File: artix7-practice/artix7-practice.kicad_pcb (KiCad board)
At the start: 2 copper layers, 20.3 x 8.4 mm, 73 parts, among them J101 USB_B_Micro, J102 Conn_02x06_Odd_Even, J103 Bus_PCI_Express_x1, Q101 Q_NMOS_GSD, U101 XC7A35T-FTG256, U104 FT2232HL, U105 93CxxC, U106 W25Q128JVS, U108 LMR33630ADDA, U109 LMR33630ADDA, U110 LMR33630ADDA, X101 125MHz, Y101 ABM8-272-T3

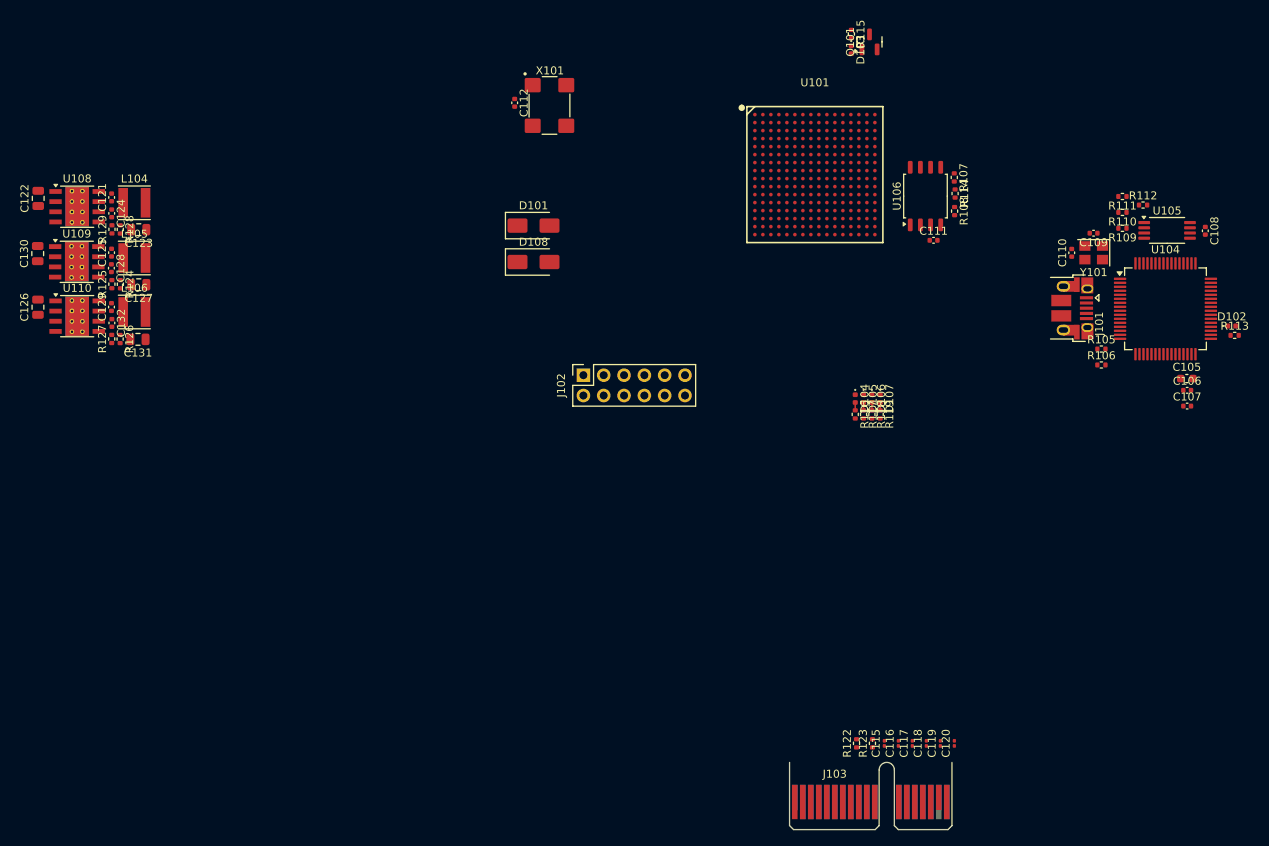
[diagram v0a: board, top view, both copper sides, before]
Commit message: JLCPCB uploads
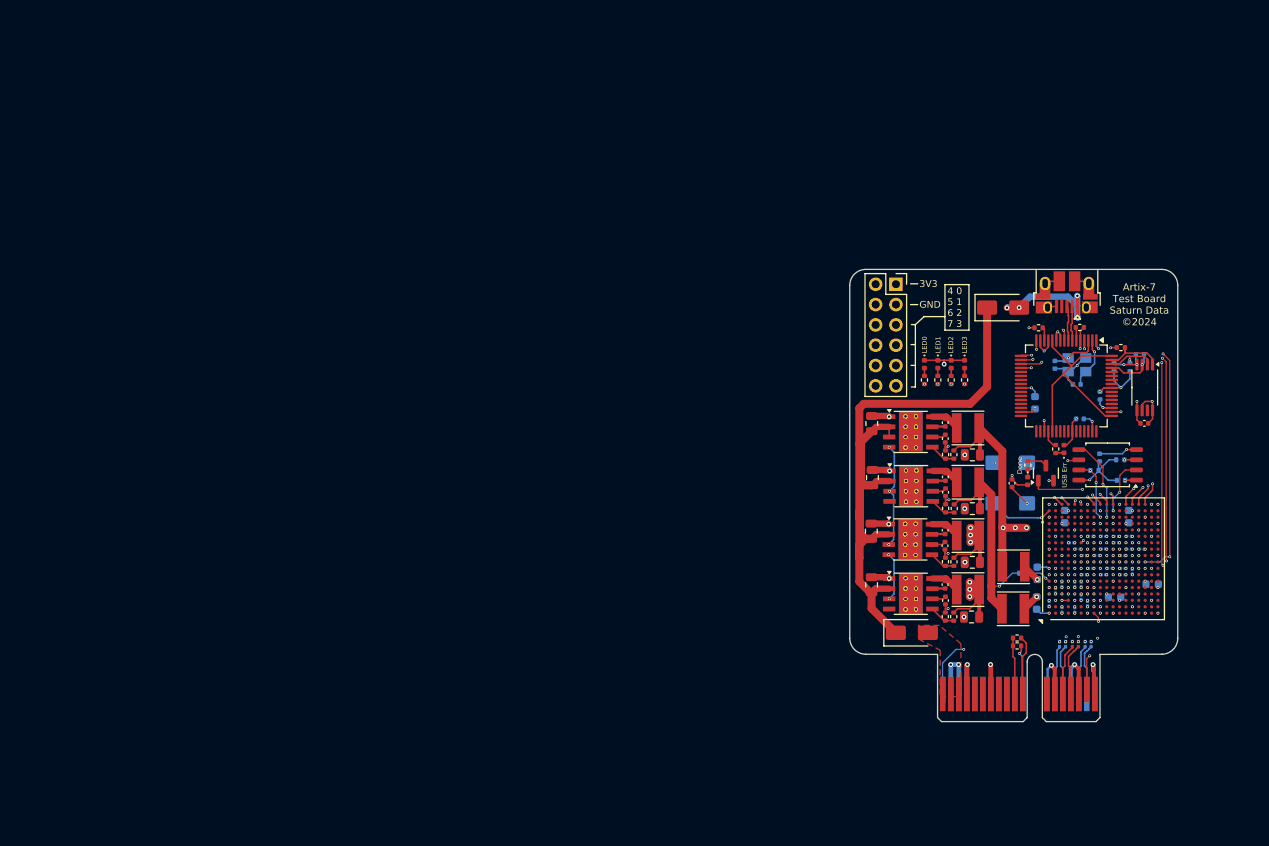
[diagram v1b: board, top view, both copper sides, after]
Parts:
- added C101: 100n, Capacitor_SMD:C_0402_1005Metric, F.Cu at (71.0, 77.8)
- added C102: 22u, Capacitor_SMD:C_0805_2012Metric, F.Cu at (61.8, 77.9)
- added C103: 22u, Capacitor_SMD:C_0805_2012Metric, F.Cu at (74.3, 81.8)
- added C104: 1u, Capacitor_SMD:C_0402_1005Metric, F.Cu at (71.0, 79.8)
- added C113: 22u, Capacitor_SMD:C_0603_1608Metric, B.Cu at (82.4, 89.9)
- added C114: 22u, Capacitor_SMD:C_0603_1608Metric, B.Cu at (82.4, 93.6)
- added C133: 1u, Capacitor_SMD:C_0201_0603Metric, B.Cu at (87.9, 91.3)
- added C134: 1u, Capacitor_SMD:C_0201_0603Metric, B.Cu at (88.7, 93.7)
- added C135: 1u, Capacitor_SMD:C_0201_0603Metric, B.Cu at (85.5, 94.5)
- added C136: 1u, Capacitor_SMD:C_0201_0603Metric, B.Cu at (84.7, 92.1)
- added C137: 1u, Capacitor_SMD:C_0201_0603Metric, B.Cu at (85.5, 91.3)
- added C138: 100n, Capacitor_SMD:C_0201_0603Metric, B.Cu at (87.1, 91.3)
- added C139: 1u, Capacitor_SMD:C_0201_0603Metric, B.Cu at (93.9, 86.9)
- added C140: 100n, Capacitor_SMD:C_0201_0603Metric, B.Cu at (87.1, 94.5)
- added C141: 100n, Capacitor_SMD:C_0201_0603Metric, B.Cu at (83.9, 93.7)
- added C142: 1u, Capacitor_SMD:C_0201_0603Metric, B.Cu at (87.9, 92.9)
- added C143: 1u, Capacitor_SMD:C_0201_0603Metric, B.Cu at (90.7, 86.9)
- added C144: 100n, Capacitor_SMD:C_0201_0603Metric, B.Cu at (93.1, 87.7)
- added C145: 100n, Capacitor_SMD:C_0201_0603Metric, B.Cu at (88.3, 87.7)
- added C146: 1u, Capacitor_SMD:C_0201_0603Metric, B.Cu at (87.5, 86.9)
- added C147: 1u, Capacitor_SMD:C_0201_0603Metric, B.Cu at (89.1, 89.3)
- added C148: 100n, Capacitor_SMD:C_0201_0603Metric, B.Cu at (93.1, 90.1)
- added C149: 100n, Capacitor_SMD:C_0201_0603Metric, B.Cu at (88.3, 90.1)
- added C150: 1u, Capacitor_SMD:C_0201_0603Metric, B.Cu at (93.1, 89.3)
- added C151: 1u, Capacitor_SMD:C_0201_0603Metric, B.Cu at (91.5, 89.3)
- added C152: 100n, Capacitor_SMD:C_0201_0603Metric, B.Cu at (90.7, 90.1)
- added C153: 100n, Capacitor_SMD:C_0201_0603Metric, B.Cu at (92.3, 86.1)
- added C154: 1u, Capacitor_SMD:C_0201_0603Metric, B.Cu at (89.1, 85.3)
- added C155: 1u, Capacitor_SMD:C_0201_0603Metric, B.Cu at (90.7, 85.3)
- added C156: 1u, Capacitor_SMD:C_0201_0603Metric, B.Cu at (93.9, 85.3)
- added C157: 100n, Capacitor_SMD:C_0201_0603Metric, B.Cu at (92.3, 85.3)
- added C158: 1u, Capacitor_SMD:C_0201_0603Metric, B.Cu at (89.9, 87.7)
- added C159: 1u, Capacitor_SMD:C_0201_0603Metric, B.Cu at (95.5, 86.9)
- added C160: 1u, Capacitor_SMD:C_0201_0603Metric, B.Cu at (86.7, 86.1)
- added C161: 1u, Capacitor_SMD:C_0201_0603Metric, B.Cu at (94.3, 89.7)
- added C162: 22u, Capacitor_SMD:C_0603_1608Metric, B.Cu at (96.8, 91.3)
- added C163: 22u, Capacitor_SMD:C_0603_1608Metric, B.Cu at (92.1, 92.9)
- added C164: 22u, Capacitor_SMD:C_0603_1608Metric, B.Cu at (85.9, 82.8)
- added C165: 22u, Capacitor_SMD:C_0603_1608Metric, B.Cu at (93.9, 82.8)
- added L101: 2.2uH, Inductor_SMD:L_Taiyo-Yuden_NR-40xx, F.Cu at (73.8, 78.5)
- added L102: 2.2uH, Inductor_SMD:L_Taiyo-Yuden_NR-40xx, F.Cu at (79.5, 89.1)
- added L103: 2.2uH, Inductor_SMD:L_Taiyo-Yuden_NR-40xx, F.Cu at (79.4, 94.3)
- added R101: 18k, Resistor_SMD:R_0402_1005Metric, F.Cu at (72.1, 81.8)
- added R102: 82k, Resistor_SMD:R_0402_1005Metric, F.Cu at (71.0, 81.8)
- added R103: 100, Resistor_SMD:R_0402_1005Metric, B.Cu at (80.7, 89.9)
- added U102: XC7A35T-CSG325, Package_BGA:Xilinx_CSG325, F.Cu at (90.7, 88.1)
- C105, C106, C107, C109, C110, C111, C115, C116, C119, C120, R107, R108, R109, R111, R112, R114, X101, Y101: moved to B.Cu
- U101: value XC7A35T-FTG256 -> LMR33630ADDA; footprint easyeda2kicad:FBGA-256_L17.0-W17.0-R16-C16-P1.00-TL -> Package_SO:Texas_HSOP-8-1EP_3.9x4.9mm_P1.27mm_ThermalVias
- moved C126 109.8 mm to (61.7, 91.3)
- moved C127 109.8 mm to (74.3, 88.5)
- moved C128 109.8 mm to (70.9, 86.4)
- moved C129 109.8 mm to (70.9, 91.3)
- moved C130 109.8 mm to (61.7, 84.6)
- moved C132 109.8 mm to (71.0, 93.3)
- moved L105 109.8 mm to (73.8, 85.2)
- moved L106 109.8 mm to (73.8, 91.9)
- moved R124 109.8 mm to (72.0, 88.5)
- moved R125 109.8 mm to (71.0, 88.4)
- moved R126 109.8 mm to (72.0, 95.3)
- moved U109 109.8 mm to (66.6, 85.7)
- moved U110 109.8 mm to (66.6, 92.4)
- moved C125 109.8 mm to (70.9, 84.5)
- moved C131 109.8 mm to (74.2, 95.3)
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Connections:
- net Net-(J103-PERn0) renamed /PCIE_TX0_PRE-
- net Net-(J103-PERp0) renamed /PCIE_TX0_PRE+
- net Net-(J103-PETn0) renamed /PCIE_RX0_PRE-
- net Net-(J103-PETp0) renamed /PCIE_RX0_PRE+
- net Net-(J103-REFCLK+) renamed /REFCLK_PRE+
- net Net-(J103-REFCLK-) renamed /REFCLK_PRE-
- D101 pad 1: /POWER -> /MAIN_PWR
- D108 pad 1: /POWER -> /MAIN_PWR
- U108 pad 4: Net-(U108-PG) -> Net-(U101-EN)
- U109 pad 3: Net-(U108-PG) -> Net-(U101-EN)
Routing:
- net GND: track 0.00 -> 99.0 mm, vias 0 -> 127
- net /MAIN_PWR: track 0.00 -> 93.6 mm
- net +1V8: track 0.00 -> 63.2 mm, vias 0 -> 9
- net +3V3: track 0.00 -> 52.5 mm, vias 0 -> 42
- net +1V0: track 0.00 -> 49.2 mm, vias 0 -> 24
- net /JTAG_TMS: track 0.00 -> 47.7 mm, vias 0 -> 4
- net /JTAG_TDI: track 0.00 -> 47.2 mm, vias 0 -> 4
- net /JTAG_TDO: track 0.00 -> 46.3 mm, vias 0 -> 4
- net /GPIO0: track 0.00 -> 43.6 mm, vias 0 -> 1
- net /GPIO4: track 0.00 -> 43.5 mm, vias 0 -> 1
- net /GPIO5: track 0.00 -> 41.2 mm, vias 0 -> 1
- net /GPIO1: track 0.00 -> 40.0 mm, vias 0 -> 1
- net /GPIO6: track 0.00 -> 39.1 mm, vias 0 -> 1
- net /LED1: track 0.00 -> 38.1 mm, vias 0 -> 2
- net /LED2: track 0.00 -> 37.1 mm, vias 0 -> 2
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- added copper zone on F.Cu, net +12V
- added copper zone on In2.Cu, net +1V0
- added copper zone on In4.Cu, net +3V3
- added copper zone on In1.Cu, net GND
- added copper zone on In3.Cu, net GND
- added copper zone on In6.Cu, net GND
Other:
- board size 20.3 x 8.4 mm -> 41 x 48.1 mm
- copper layers 2 -> 8
- board text added: "3V3"
- board text added: "4 0 5 1 6 2 7 3"
- board text added: "Artix-7 Test Board Peter Schmidt-Nielsen Saturn Data"
- board text added: "Artix-7 Test Board Saturn Data ©2024"
- board text added: "Done"
- board text added: "GND"
- board text added: "LED0"
- board text added: "LED1"
- board text added: "LED2"
- board text added: "LED3"
- board text added: "USB Err"
